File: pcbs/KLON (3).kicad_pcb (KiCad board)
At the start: 2 copper layers, 159.6 x 117.7 mm, 83 parts

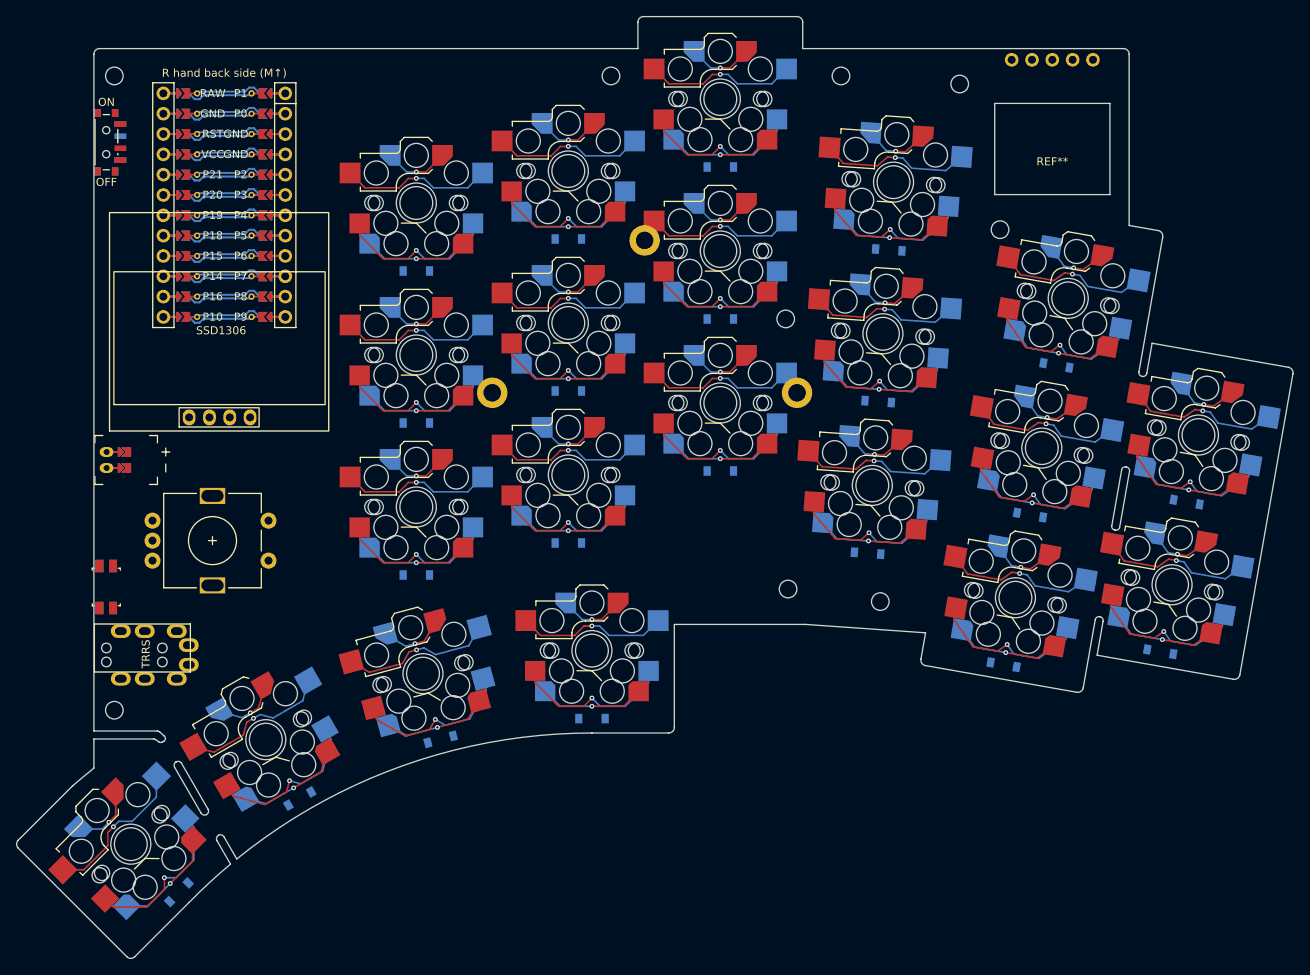
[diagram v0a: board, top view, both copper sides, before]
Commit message: pcb changes
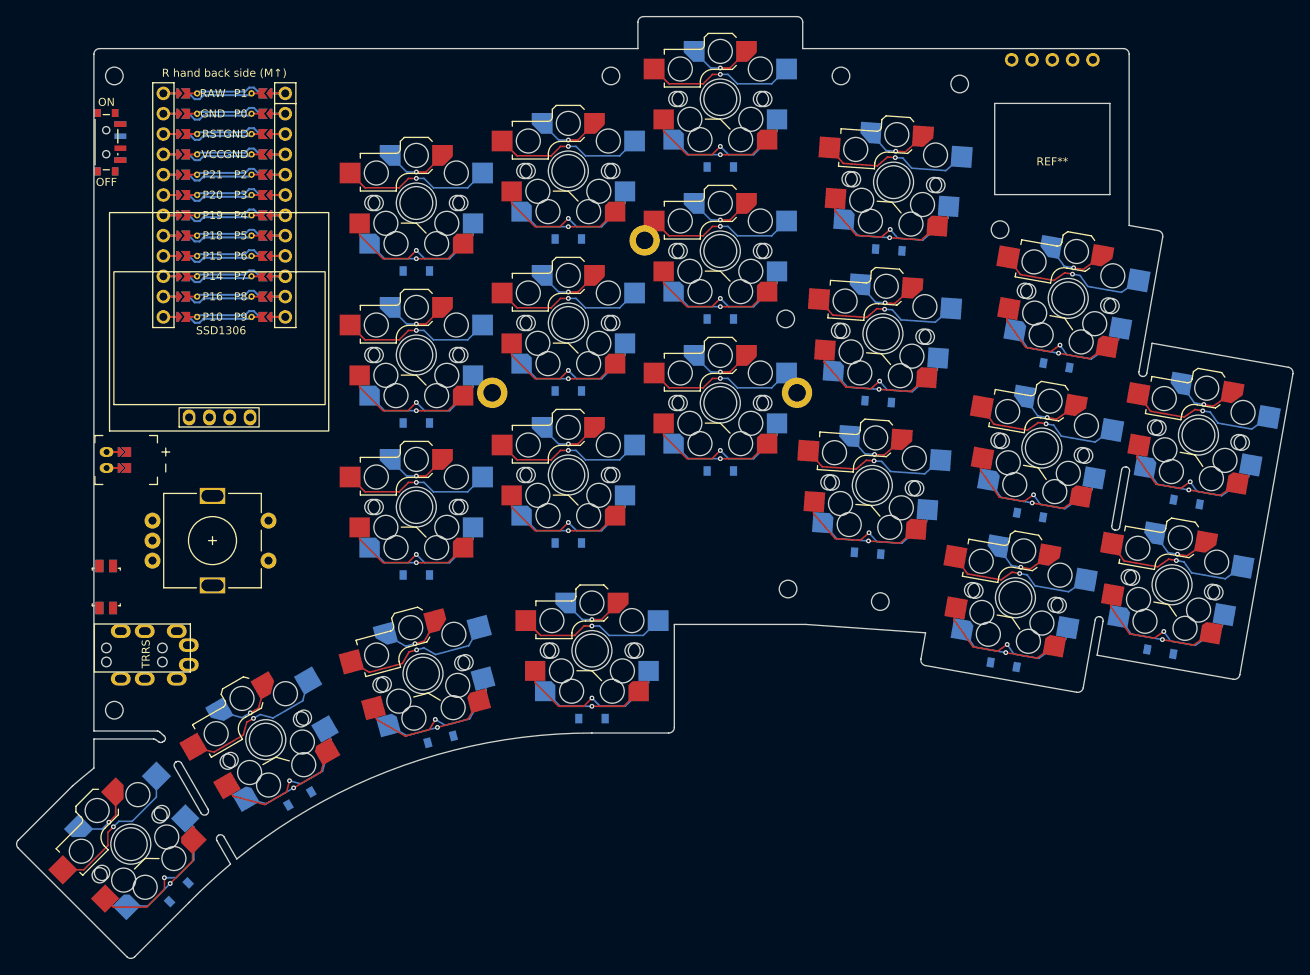
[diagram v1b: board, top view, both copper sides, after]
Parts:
- removed XX1: , Pimoroni Haptic Buzz DRV2605L Driver
- removed XX2: , RotaryEncoder_Alps_EC11E-Switch_Vertical_H20mm-keebio_modified
- removed XX3: , SSD1306_128x64OLED
- removed XX4: , MJ-4PP-9
- added J1: MJ-4PP-9, MJ-4PP-9, F.Cu at (129.8, 167.6)
- added REF**: Pimoroni Haptic Buzz DRV2605L Driver, Pimoroni Haptic Buzz DRV2605L Driver, F.Cu at (249.5, 104.5)
- added SSD1306: SSD1306_128x64OLED, SSD1306_128x64OLED, F.Cu at (145.6, 128.2)
- added SW25: Rotary_Encoder_Switch, RotaryEncoder_Alps_EC11E-Switch_Vertical_H20mm-keebio_modified, F.Cu at (144.5, 154.2)
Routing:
- net (no net): track 733.6 -> 173.6 mm, vias 42 -> 21
- net GND: track 0.00 -> 29.5 mm
- net pinky_bottom: track 42.2 -> 52.7 mm, vias 2 -> 3
- net 2_r0: track 42.2 -> 52.7 mm, vias 2 -> 3
- net 3_r0: track 42.2 -> 52.7 mm, vias 2 -> 3
- net middle_top: track 42.2 -> 52.7 mm, vias 2 -> 3
- net middle_home: track 42.2 -> 52.7 mm, vias 2 -> 3
- net middle_bottom: track 42.2 -> 52.7 mm, vias 2 -> 3
- net inner_top: track 42.2 -> 52.7 mm, vias 2 -> 3
- net inner_home: track 42.2 -> 52.7 mm, vias 2 -> 3
- net inner_bottom: track 42.2 -> 52.7 mm, vias 2 -> 3
- net index_top: track 42.2 -> 52.7 mm, vias 2 -> 3
- net index_bottom: track 42.2 -> 52.7 mm, vias 2 -> 3
- net index_home: track 42.2 -> 52.7 mm, vias 2 -> 3
- net 1_r0: track 42.2 -> 52.7 mm, vias 2 -> 3
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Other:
- outline, holes or cut-outs redrawn
